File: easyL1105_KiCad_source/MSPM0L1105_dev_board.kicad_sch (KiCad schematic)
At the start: 51 parts, among them J1 IO_A, J2 IO_B, J3 UART-SELECT, J4 USB_C_Receptacle_USB4085, J5 SWD, J6 LDO_JUMPER, J7 GND_JUMPER, SW1 RESET, SW2 BSL_BOOT, SW3 USER_PA16, U1 MSPM0L1105TDGS28R, U2 CH340K, U3 SRV05-4, U4 MIC5209-3.3YS

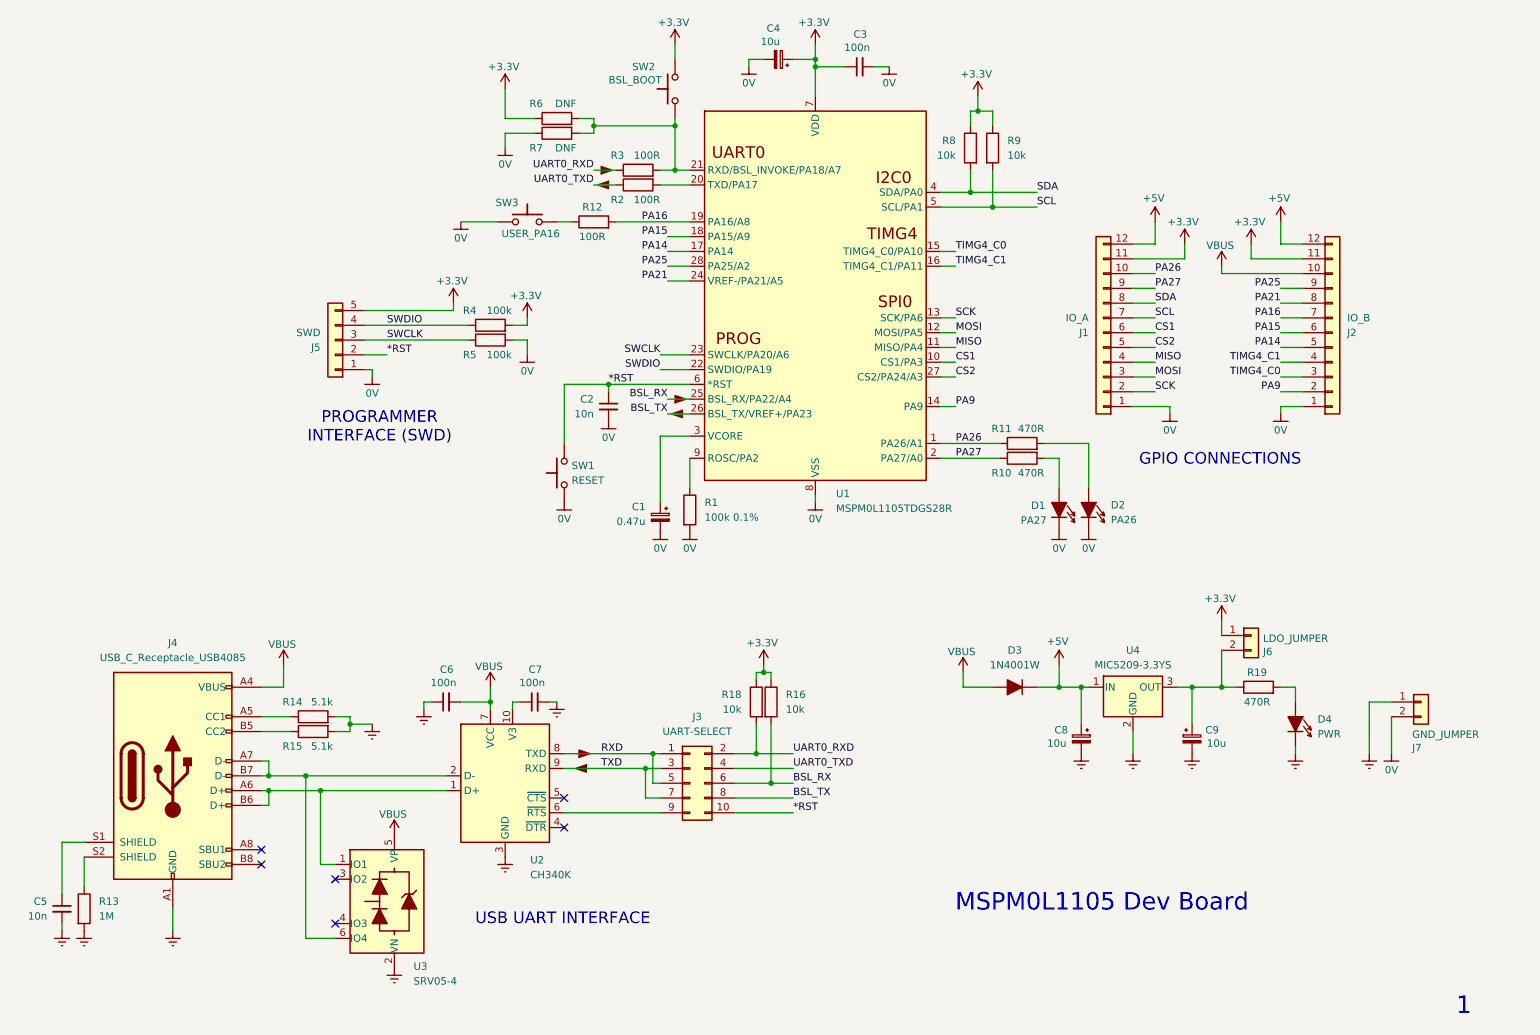
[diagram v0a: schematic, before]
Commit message: Add files via upload
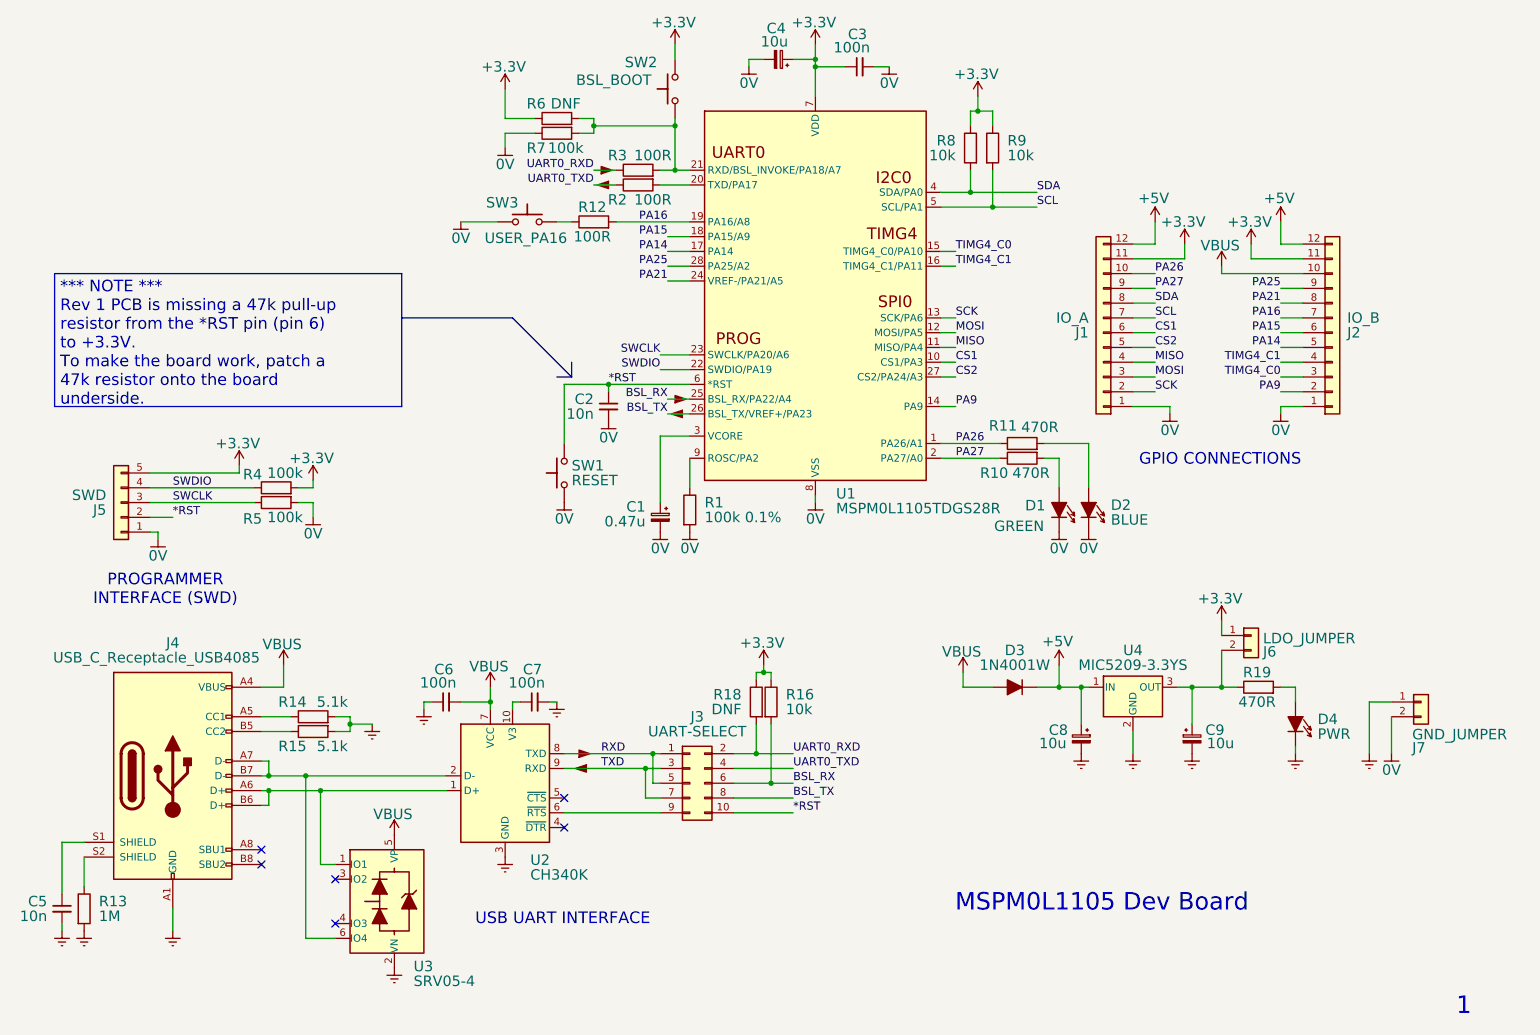
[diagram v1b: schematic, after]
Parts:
- D1: value PA27 -> GREEN
- D2: value PA26 -> BLUE
- R18: value 10k -> DNF
- R7: value DNF -> 100k
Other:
- moved on the sheet: J5, R4, R5
